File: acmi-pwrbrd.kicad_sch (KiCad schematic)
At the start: 25 parts, among them J1 430450402, J10 3-641215-8, J2 430450402, J3 430451202, J4 430451202, J5 430450402

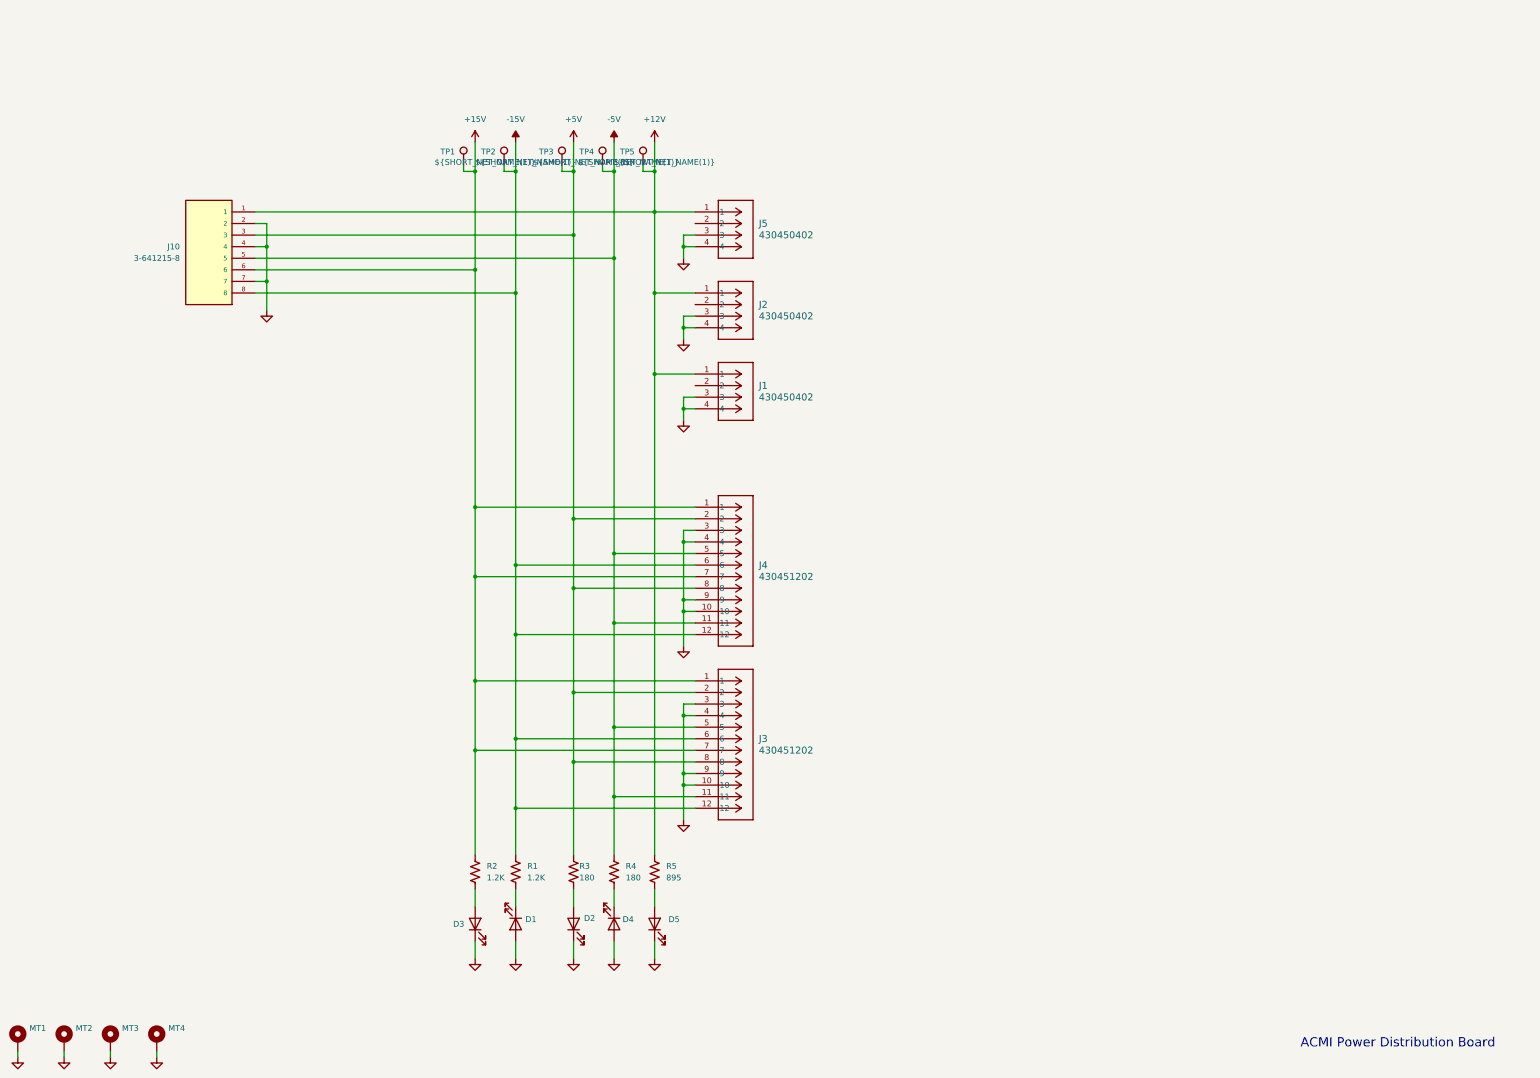
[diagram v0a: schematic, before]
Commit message: Finish routing
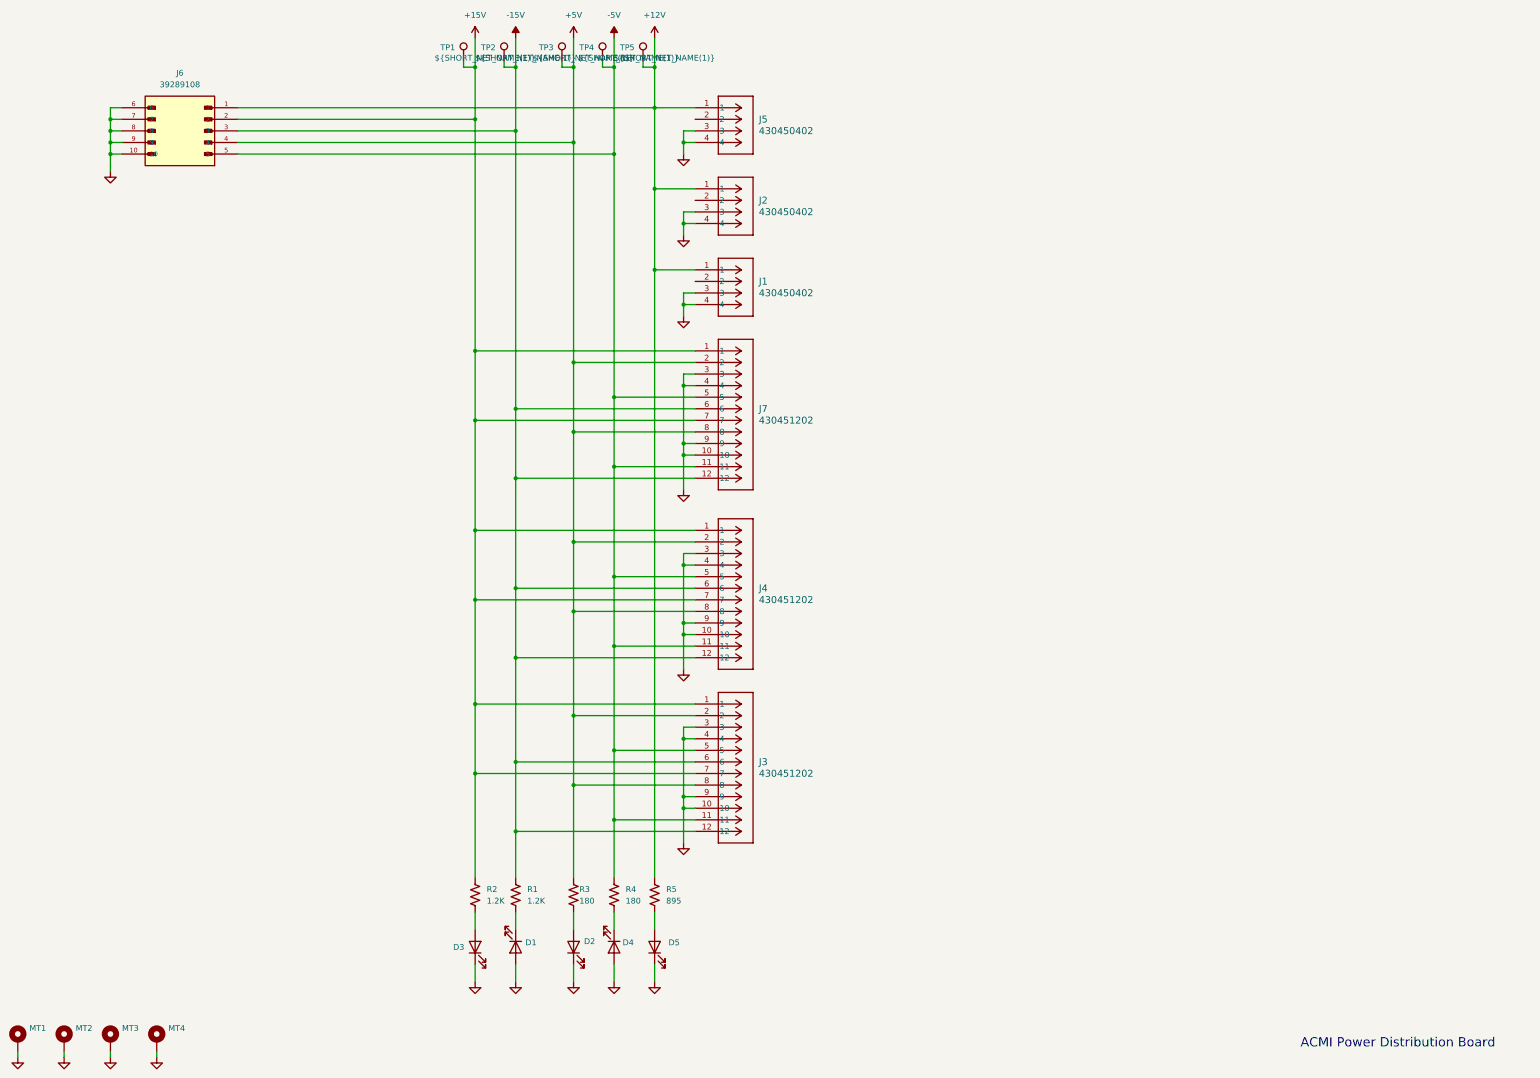
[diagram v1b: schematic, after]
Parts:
- removed J10: 3-641215-8, 3-641215-8:TE_3-641215-8, symbol myparts:3-641215-8
- added J6: 39289108, myparts:MOLEX_39289108, symbol myparts:39289108
- added J7: 430451202, myparts:CONN_SD-43045-001_12_MOL, symbol myparts:430451202
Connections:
- net +12V: now also J6.1
- net +15V: now also J6.2, J7.1, J7.7
- net +5V: now also J6.4, J7.2, J7.8
- net -15V: now also J6.3, J7.12, J7.6
- net -5V: now also J6.5, J7.11, J7.5
- net GND: now also J6.10, J6.6, J6.7, J6.8, J6.9, J7.10, J7.3, J7.4, J7.9
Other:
- moved on the sheet: D1, D2, D3, D4, D5, J1, J2, J3, J4, J5, R1, R2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
